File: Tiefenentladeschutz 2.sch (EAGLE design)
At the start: 37 parts, among them IC1 ICL7665CSA, IC2 NE555D, T2 BCV26 PNP

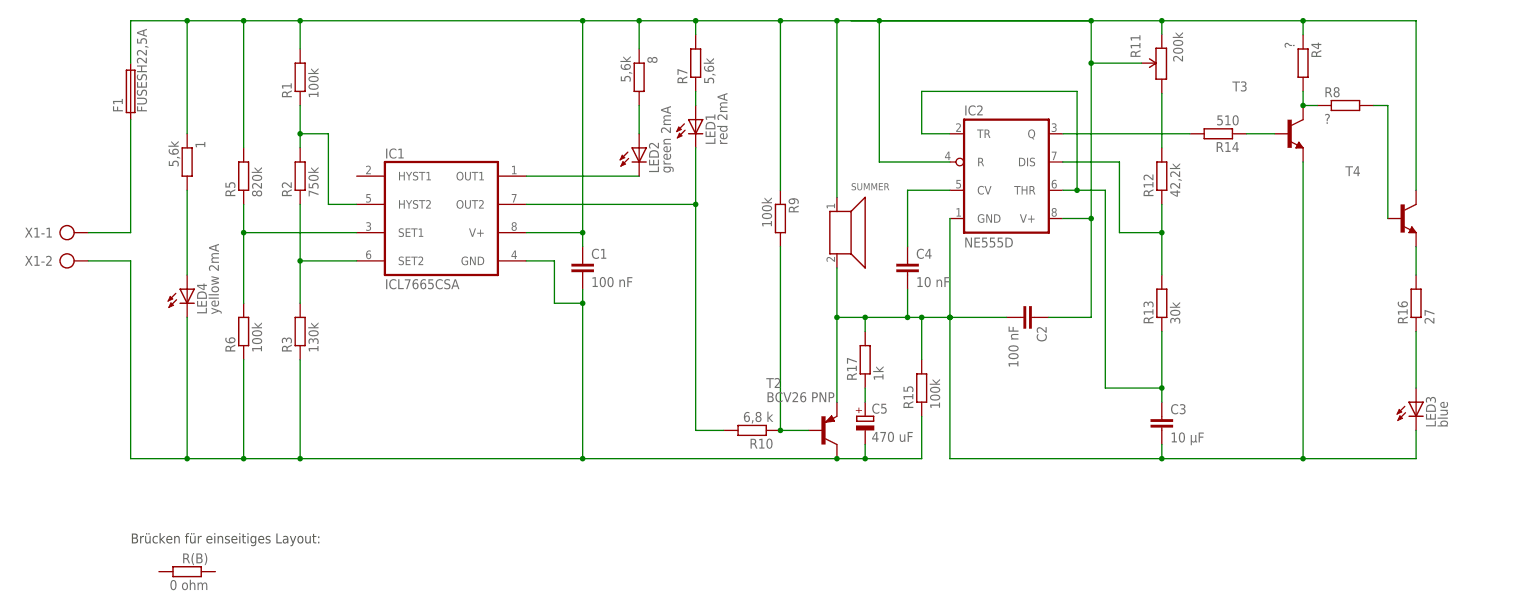
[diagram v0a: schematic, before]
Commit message: v2.4
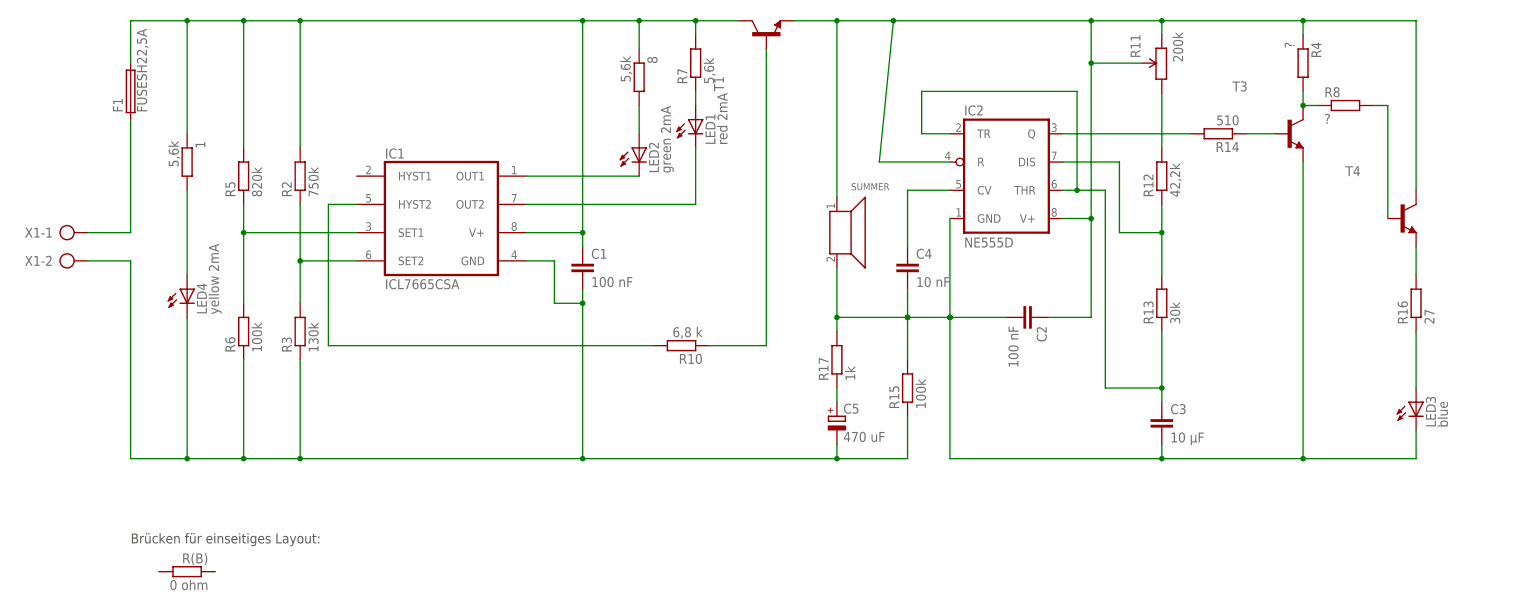
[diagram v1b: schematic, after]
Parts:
- removed R1, R9: 100k, eagle-ltspice:RR1206
- removed T2: BCV26 PNP, transistor:-PNP-SOT23-BCE
- added T1: (no value), transistor:BC817-40-NPN-SOT23-BEC
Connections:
- new net N$26: 1.1, 8.1, C1.1, F1.2, IC1.V+, R2.2, R5.2, R7.2, T1.C
- net GND: no longer T2.C
- net N$1: now also R10.2; no longer R1.1, R2.2
- net N$10: no longer R10.2
- net N$22: no longer T2.E
- net N$7: now also T1.B; no longer R9.2, T2.B
- net V+: now also T1.E; no longer 1.1, 8.1, C1.1, F1.2, IC1.V+, R1.2, R5.2, R7.2, R9.1
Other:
- moved on the sheet: C5, R10, R15, R17

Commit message: 2.6
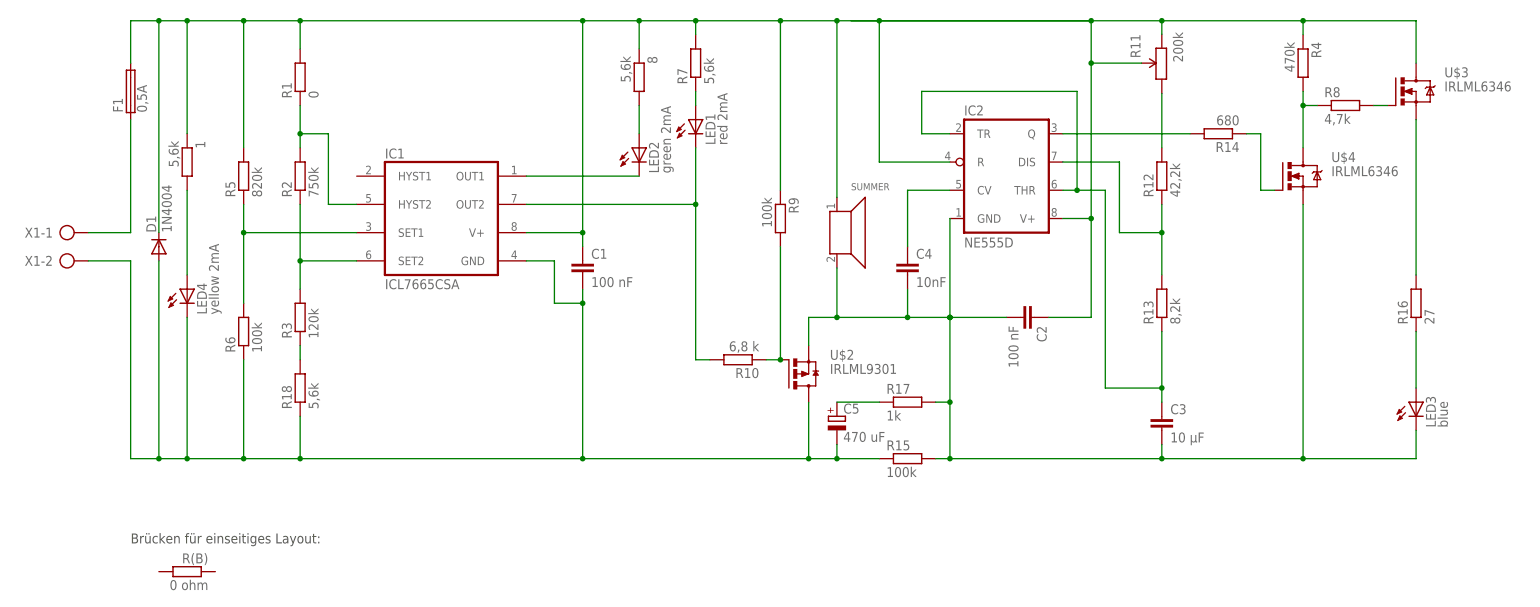
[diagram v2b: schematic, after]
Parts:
- removed T1, T3, T4: (no value), transistor:BC817-40-NPN-SOT23-BEC
- added D1: 1N4004, diode:1N4004
- added R1: 0, eagle-ltspice:RR1206
- added R18: 5,6k, eagle-ltspice:RR1206
- added R9: 100k, eagle-ltspice:RR1206
- added U$2: IRLML9301, 0liver:IRLML9301
- added U$3, U$4: IRLML6346, 0liver:IRLML6346
- C4: value 10 nF -> 10nF; device eagle-ltspice:CC1206 -> rcl:C-EUC0805K
- F1: value FUSESH22,5A -> 0,5A
- R13: value 30k -> 8,2k
- R14: value 510 -> 680
- R3: value 130k -> 120k
- R4: value ? -> 470k
- R8: value ? -> 4,7k
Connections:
- net GND: now also D1.A, R18.1, U$2.D; no longer R3.1
- net N$1: now also R1.1, R2.2; no longer R10.2
- net N$10: now also R10.2
- net N$17: now also U$3.G; no longer T4.B
- net N$18: now also U$4.G; no longer T3.B
- net N$21: now also U$4.D; no longer T3.C
- net N$22: now also U$2.S, U$4.S; no longer T3.E
- net N$26: now also R18.2, R3.1; no longer 1.1, 8.1, C1.1, F1.2, IC1.V+, R2.2, R5.2, R7.2, T1.C
- net N$3: now also U$3.S; no longer T4.E
- net N$7: now also R9.2, U$2.G; no longer T1.B
- net V+: now also 1.1, 8.1, C1.1, D1.C, F1.2, IC1.V+, R1.2, R5.2, R7.2, R9.1, U$3.D; no longer T1.E, T4.C
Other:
- moved on the sheet: R10, R15, R17, R3
